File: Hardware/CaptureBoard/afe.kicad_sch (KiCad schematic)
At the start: 41 parts, among them U1 ADA4800, U2 ADA4800, U800 AD9990, Y800 30MHz

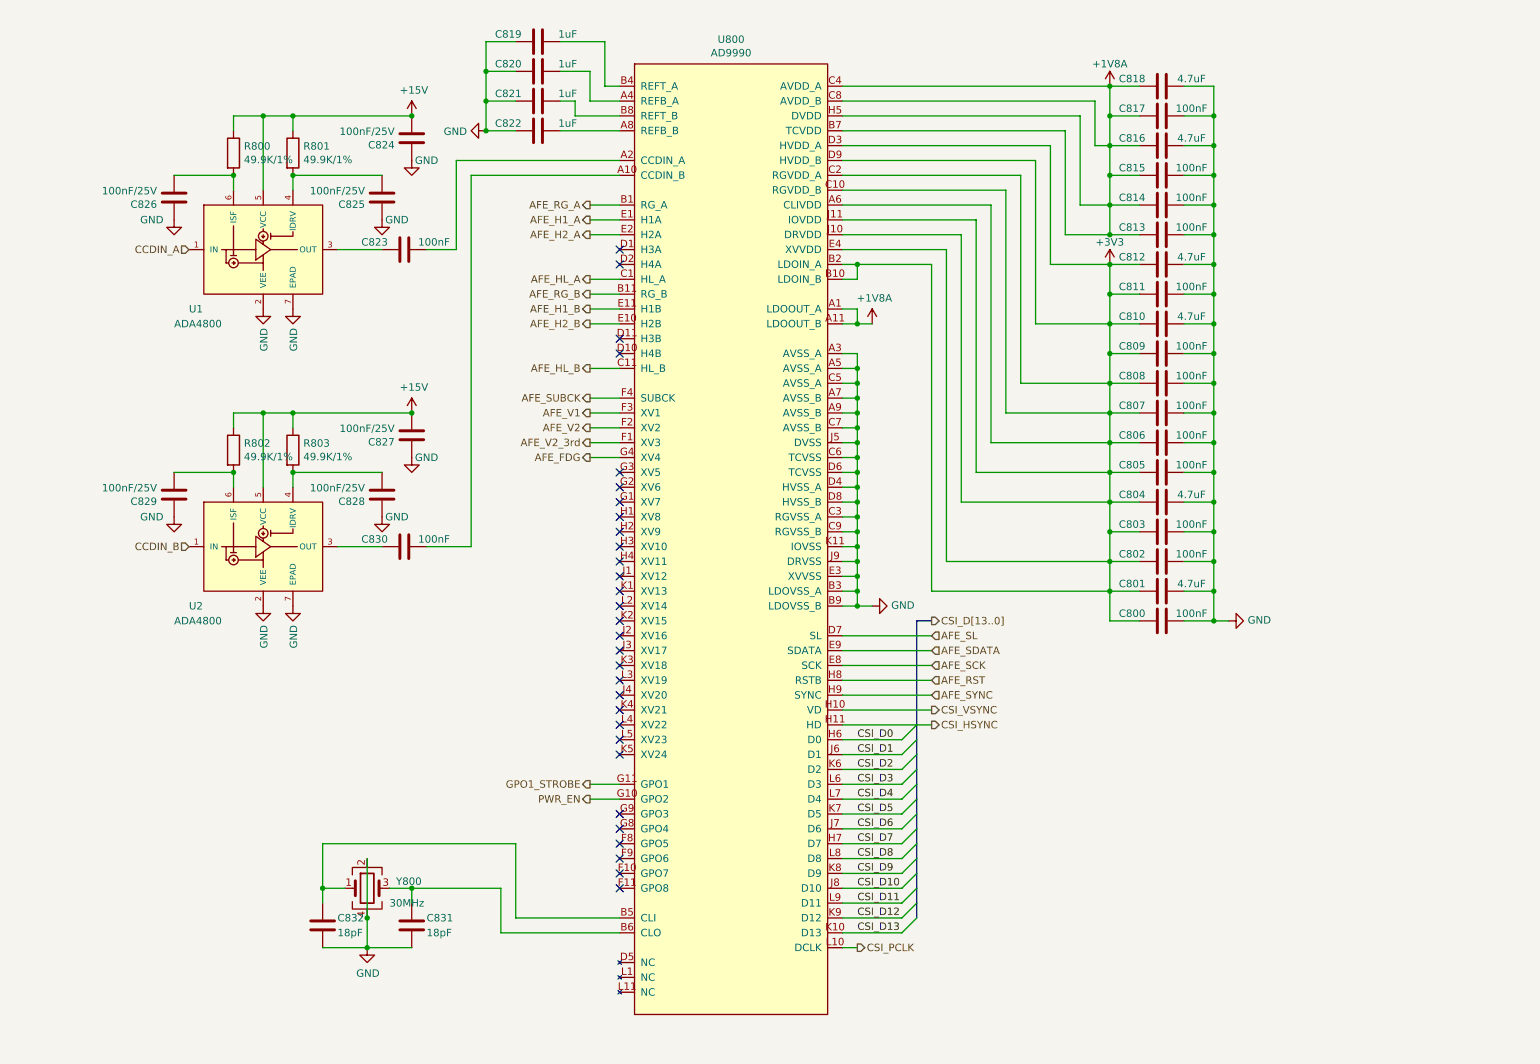
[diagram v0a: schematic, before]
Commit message: pcb: switch to ad9978 wip
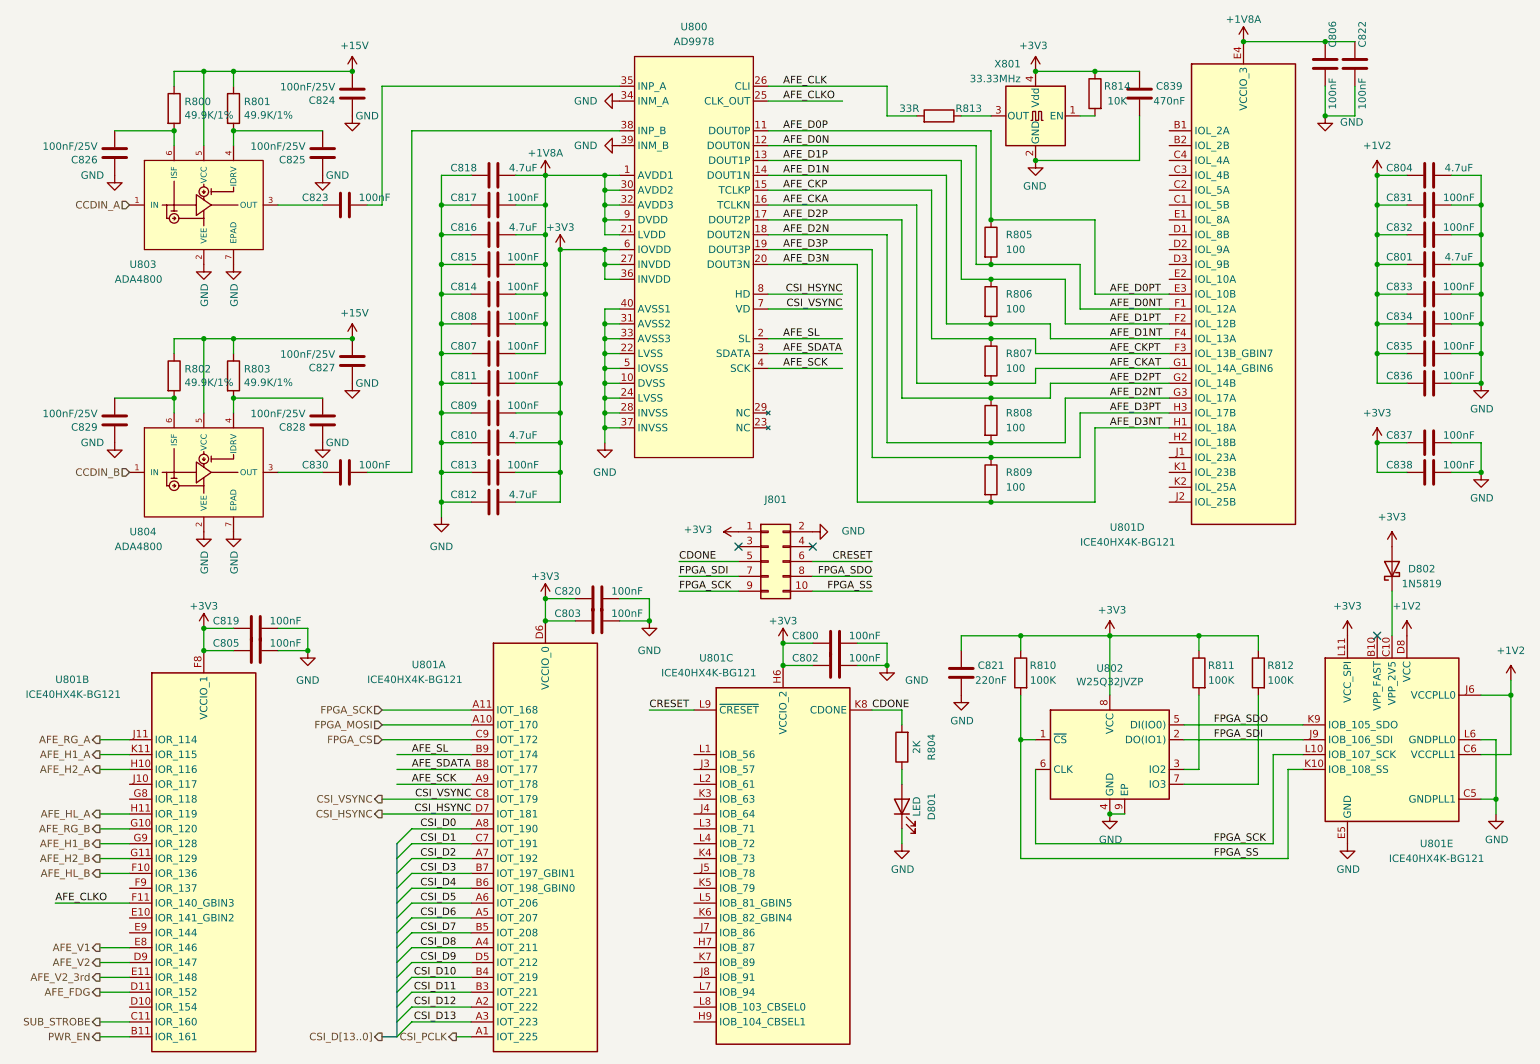
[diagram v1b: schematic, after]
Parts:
- removed U800: AD9990, Footprints:BGA-112_11x11_8.0x8.0mm, symbol Sitina:AD9990
- removed Y800: 30MHz, Crystal:Crystal_SMD_3225-4Pin_3.2x2.5mm, symbol Device:Crystal_GND24
- added C833, C834, C835, C836, C837, C838: 100nF, Capacitor_SMD:C_0402_1005Metric, symbol Device:C
- added C839: 470nF, Capacitor_SMD:C_0402_1005Metric, symbol Device:C
- added D801: LED, Diode_SMD:D_0603_1608Metric, symbol Device:LED
- added D802: 1N5819, Diode_SMD:D_SOD-123, symbol Diode:MBR0530
- added J801: Conn_02x05_Odd_Even, Connector_PinHeader_1.27mm:PinHeader_2x05_P1.27mm_Vertical_SMD, symbol Connector_Generic:Conn_02x05_Odd_Even
- added R804: 2K, Resistor_SMD:R_0402_1005Metric, symbol Device:R
- added R805, R806, R807, R808, R809: 100, Resistor_SMD:R_0402_1005Metric, symbol Device:R
- added R810, R811, R812: 100K, Resistor_SMD:R_0402_1005Metric, symbol Device:R
- added R813: 33R, Capacitor_SMD:C_0402_1005Metric, symbol Device:R
- added R814: 10K, Capacitor_SMD:C_0402_1005Metric, symbol Device:R
- added U800: AD9978, Package_DFN_QFN:QFN-40-1EP_6x6mm_P0.5mm_EP4.6x4.6mm, symbol Sitina:AD9978
- added U801: ICE40HX4K-BG121, Package_BGA:BGA-121_9.0x9.0mm_Layout11x11_P0.8mm_Ball0.4mm_Pad0.35mm_NSMD, symbol FPGA_Lattice:ICE40HX4K-BG121
- added U802: W25Q32JVZP, Package_SON:WSON-8-1EP_6x5mm_P1.27mm_EP3.4x4.3mm, symbol Memory_Flash:W25Q32JVZP
- added X801: 33.33MHz, Oscillator:Oscillator_SMD_Abracon_ASE-4Pin_3.2x2.5mm, symbol Oscillator:ASE-xxxMHz
- C819, C820, C822: value 1uF -> 100nF
- C821: value 1uF -> 220nF
- C831, C832: value 18pF -> 100nF; footprint Capacitor_SMD:C_0603_1608Metric -> Capacitor_SMD:C_0402_1005Metric
- U803: renamed from U1; footprint Package_DFN_QFN:DFN-6-1EP_2x1.8mm_P0.5mm_EP1.2x1.6mm -> Package_DFN_QFN:DFN-6-1EP_2x2mm_P0.5mm_EP0.6x1.37mm
- U804: renamed from U2; footprint Package_DFN_QFN:DFN-6-1EP_2x1.8mm_P0.5mm_EP1.2x1.6mm -> Package_DFN_QFN:DFN-6-1EP_2x2mm_P0.5mm_EP0.6x1.37mm
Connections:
- net +1V8A: now also C806.2, C807.1, C808.1, C814.1, C815.1, C816.1, C817.1, C818.1, C822.2, U800.1 (AVDD1), U800.21 (LVDD), U800.30 (AVDD2), U800.32 (AVDD3), U800.9 (DVDD), U801.E4 (VCCIO_3), U801.G4 (VCCIO_3); no longer C813.2, C814.2, C815.2, C816.2, C817.2, C818.2
- net +3V3: now also C809.1, C810.1, C811.1, C812.1, C813.1, C819.2, C820.2, C821.2, C837.2, C838.2, C839.2, D802.2 (A), J801.1 (Pin_1), R810.1, R811.1, R812.1, R814.1, U800.27 (INVDD), U800.36 (INVDD), U800.6 (IOVDD), U801.D6 (VCCIO_0), U801.F8 (VCCIO_1), U801.H6 (VCCIO_2), U801.L11 (VCC_SPI), U802.8 (VCC), X801.4 (Vdd); no longer C801.2, C804.2, C806.2, C807.2, C808.2, C809.2, C810.2, C811.2, C812.2
- net AFE_FDG: now also U801.D11 (IOR_152)
- net AFE_H1_A: now also U801.K11 (IOR_115)
- net AFE_H1_B: now also U801.G9 (IOR_128)
- net AFE_H2_A: now also U801.H10 (IOR_116)
- net AFE_H2_B: now also U801.G11 (IOR_129)
- net AFE_HL_A: now also U801.H11 (IOR_119)
- net AFE_HL_B: now also U801.F10 (IOR_136)
- net AFE_RG_A: now also U801.J11 (IOR_114)
- net AFE_RG_B: now also U801.G10 (IOR_120)
- net AFE_SCK: now also U800.4 (SCK), U801.A9 (IOT_178)
- net AFE_SDATA: now also U800.3 (SDATA), U801.B8 (IOT_177)
- net AFE_SL: now also U800.2 (SL), U801.B9 (IOT_174)
- net AFE_V1: now also U801.E8 (IOR_146)
- net AFE_V2: now also U801.D9 (IOR_147)
- net AFE_V2_3rd: now also U801.E11 (IOR_148)
- net CSI_D0: now also U801.A8 (IOT_190)
- net CSI_D1: now also U801.C7 (IOT_191)
- net CSI_D10: now also U801.B4 (IOT_219)
- net CSI_D11: now also U801.B3 (IOT_221)
- net CSI_D12: now also U801.A2 (IOT_222)
- net CSI_D13: now also U801.A3 (IOT_223)
- net CSI_D2: now also U801.A7 (IOT_192)
- net CSI_D3: now also U801.B7 (IOT_197_GBIN1)
- net CSI_D4: now also U801.B6 (IOT_198_GBIN0)
- net CSI_D5: now also U801.A6 (IOT_206)
- net CSI_D6: now also U801.A5 (IOT_207)
- net CSI_D7: now also U801.B5 (IOT_208)
- net CSI_D8: now also U801.A4 (IOT_211)
- net CSI_D9: now also U801.D5 (IOT_212)
- net CSI_HSYNC: now also U800.8 (HD), U801.D7 (IOT_181)
- net CSI_PCLK: now also U801.A1 (IOT_225)
- net CSI_VSYNC: now also U800.7 (VD), U801.C8 (IOT_179)
- net GND: now also C807.2, C808.2, C809.2, C810.2, C811.2, C812.2, C813.2, C814.2, C815.2, C816.2, C817.2, C818.2, C819.1, C820.1, C821.1, C822.1, C833.1, C834.1, C835.1, C836.1, C837.1, C838.1, C839.1, D801.1 (K), J801.2 (Pin_2), U800.10 (DVSS), U800.22 (LVSS), U800.24 (LVSS), U800.28 (INVSS), U800.31 (AVSS2), U800.33 (AVSS3), U800.34 (INM_A), U800.37 (INVSS), U800.39 (INM_B), U800.40 (AVSS1), U800.5 (IOVSS), U801.C5 (GNDPLL1), U801.E5 (GND), U801.E6 (GND), U801.E7 (GND), U801.F5 (GND), U801.F6 (GND), U801.F7 (GND), U801.G5 (GND), U801.G6 (GND), U801.G7 (GND), U801.H5 (GND), U801.L6 (GNDPLL0), U802.4 (GND), U802.9 (EP), X801.2 (GND); no longer C807.1, C808.1, C809.1, C810.1, C811.1, C812.1, C813.1, C814.1, C815.1, C816.1, C817.1, C818.1, C819.2, C820.2, C821.2, C822.2
- net PWR_EN: now also U801.B11 (IOR_161)
- net at C830.1: now also U800.38 (INP_B)
- net at C823.1: now also U800.35 (INP_A)
- net +1V2: now reaches C832.2
- net +1V2: now also C801.2, C804.2, C831.2, C833.2, C834.2, C835.2, C836.2, U801.C6 (VCCPLL1), U801.D4 (VCC), U801.D8 (VCC), U801.H4 (VCC), U801.H8 (VCC), U801.J6 (VCCPLL0)
- new net: R811.2, U802.3 (IO2)
- new net: R812.2, U802.7 (IO3)
- new net: D801.2 (A), R804.1
- new net: D802.1 (K), U801.C10 (VPP_2V5)
- new net: R814.2, X801.1 (EN)
- new net: R813.1, X801.3 (OUT)
- new net AFE_CKA: R807.2, U800.16 (TCLKN), U801.G1 (IOL_14A_GBIN6)
- new net AFE_CKP: R807.1, U800.15 (TCLKP), U801.F3 (IOL_13B_GBIN7)
- new net AFE_CLK: R813.2, U800.26 (CLI)
- new net AFE_CLKO: U800.25 (CLK_OUT), U801.F11 (IOR_140_GBIN3)
- new net AFE_D0N: R805.2, U800.12 (DOUT0N), U801.F1 (IOL_12A)
- new net AFE_D0P: R805.1, U800.11 (DOUT0P), U801.E3 (IOL_10B)
- new net AFE_D1N: R806.2, U800.14 (DOUT1N), U801.F4 (IOL_13A)
- new net AFE_D1P: R806.1, U800.13 (DOUT1P), U801.F2 (IOL_12B)
- new net AFE_D2N: R808.2, U800.18 (DOUT2N), U801.G3 (IOL_17A)
- new net AFE_D2P: R808.1, U800.17 (DOUT2P), U801.G2 (IOL_14B)
- new net AFE_D3N: R809.2, U800.20 (DOUT3N), U801.H1 (IOL_18A)
- new net AFE_D3P: R809.1, U800.19 (DOUT3P), U801.H3 (IOL_17B)
- new net CDONE: J801.5 (Pin_5), R804.2, U801.K8 (CDONE)
- new net CRESET: J801.6 (Pin_6), U801.L9 (~{CRESET})
- new net FPGA_CS: U801.C9 (IOT_172)
- new net FPGA_MOSI: U801.A10 (IOT_170)
- new net FPGA_SCK: J801.9 (Pin_9), U801.A11 (IOT_168), U801.L10 (IOB_107_SCK), U802.6 (CLK)
- new net FPGA_SDI: J801.7 (Pin_7), U801.J9 (IOB_106_SDI), U802.2 (DO(IO1))
- new net FPGA_SDO: J801.8 (Pin_8), U801.K9 (IOB_105_SDO), U802.5 (DI(IO0))
- new net FPGA_SS: J801.10 (Pin_10), R810.2, U801.K10 (IOB_108_SS), U802.1 (~{CS})
- new net SUB_STROBE: U801.C11 (IOR_160)
- no-connect marks 30 -> 3
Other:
- moved on the sheet: C800, C801, C802, C803, C804, C805, C806, C807, C808, C809, C810, C811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
